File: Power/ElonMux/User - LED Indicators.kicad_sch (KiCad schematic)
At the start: 5 parts, among them Q1101 PMV90ENER

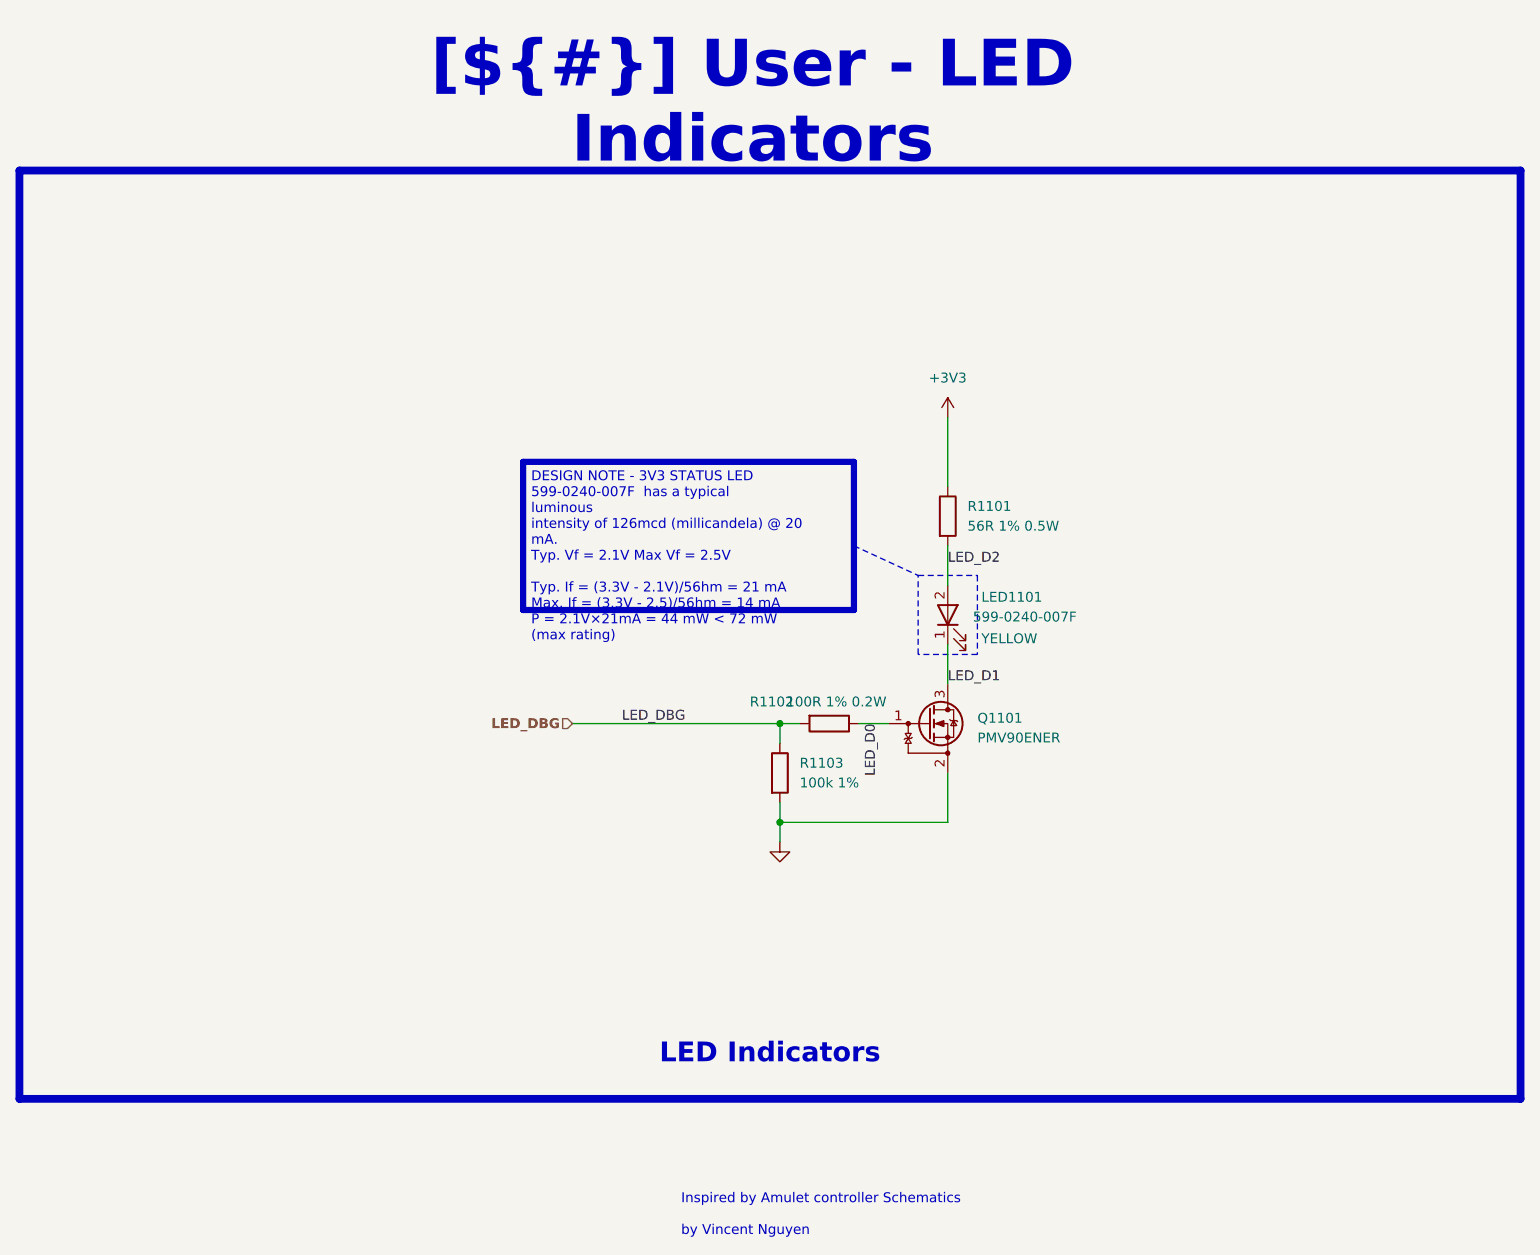
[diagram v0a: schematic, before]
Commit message: Merged ElonMux v1.0
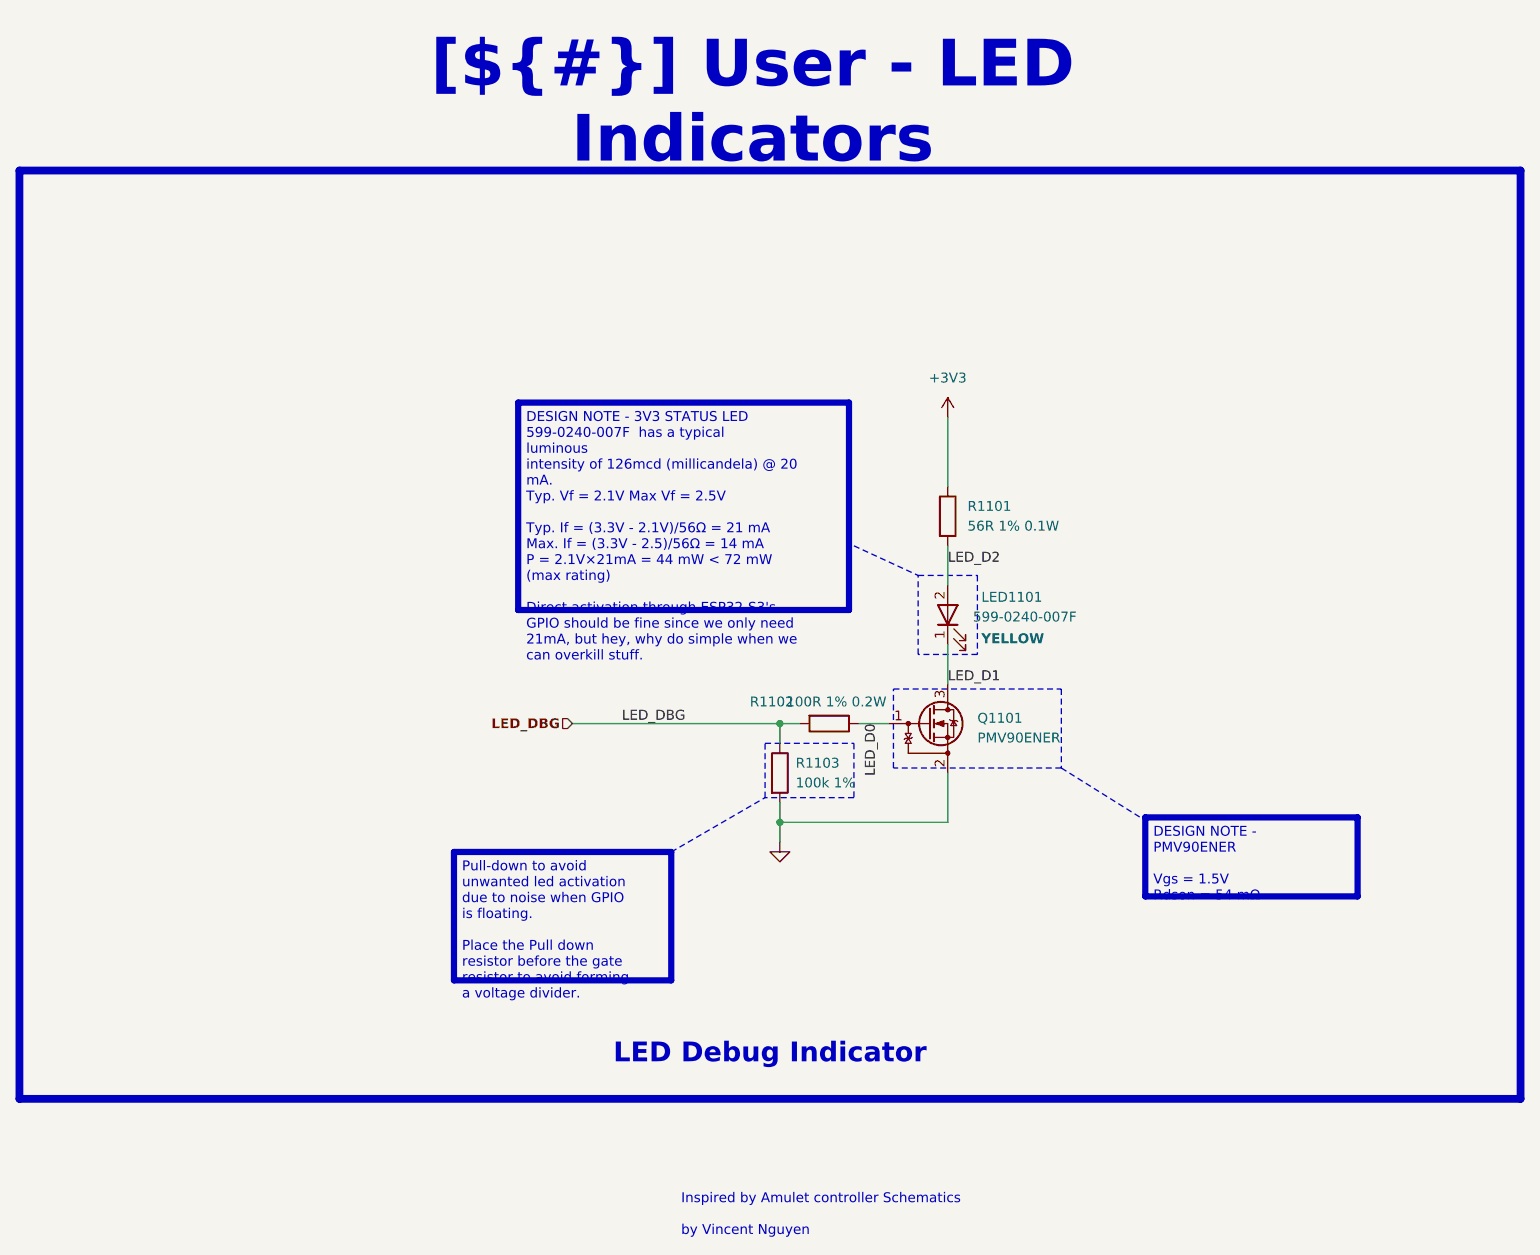
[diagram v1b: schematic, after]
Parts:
- R1101: value 56R 1% 0.5W -> 56R 1% 0.1W; footprint Resistor_SMD:R_0805_2012Metric_Pad1.20x1.40mm_HandSolder -> Resistor_SMD:R_0402_1005Metric; Manufacturer KOA Speer -> Panasonic; Manufacturer Part Number SG73P2ATTD56R0F -> ERJ-2RKF56R0X; Supplier Part Number 660-SG73P2ATTD56R0F -> 667-ERJ-2RKF56R0X
- R1103: Manufacturer Part Number ERJ-PA2F1003X -> ERJ-2RKF1003X; Supplier Part Number 667-ERJ-PA2F1003X -> 667-ERJ-2RKF1003X
